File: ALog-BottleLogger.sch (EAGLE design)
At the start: 103 parts, among them IC2 ATMEGA644M, J6 5.5x2.1mm Barrel, Q1 220mA/50V/3.5Ω, Q4 4.3A/20V/54mΩ, Q5 4.3A/20V/54mΩ, Q6 4.3A/20V/54mΩ, Q7 4.3A/20V/54mΩ, Q8 220mA/50V/3.5Ω, Q9 220mA/50V/3.5Ω, U2 FT231X-Q

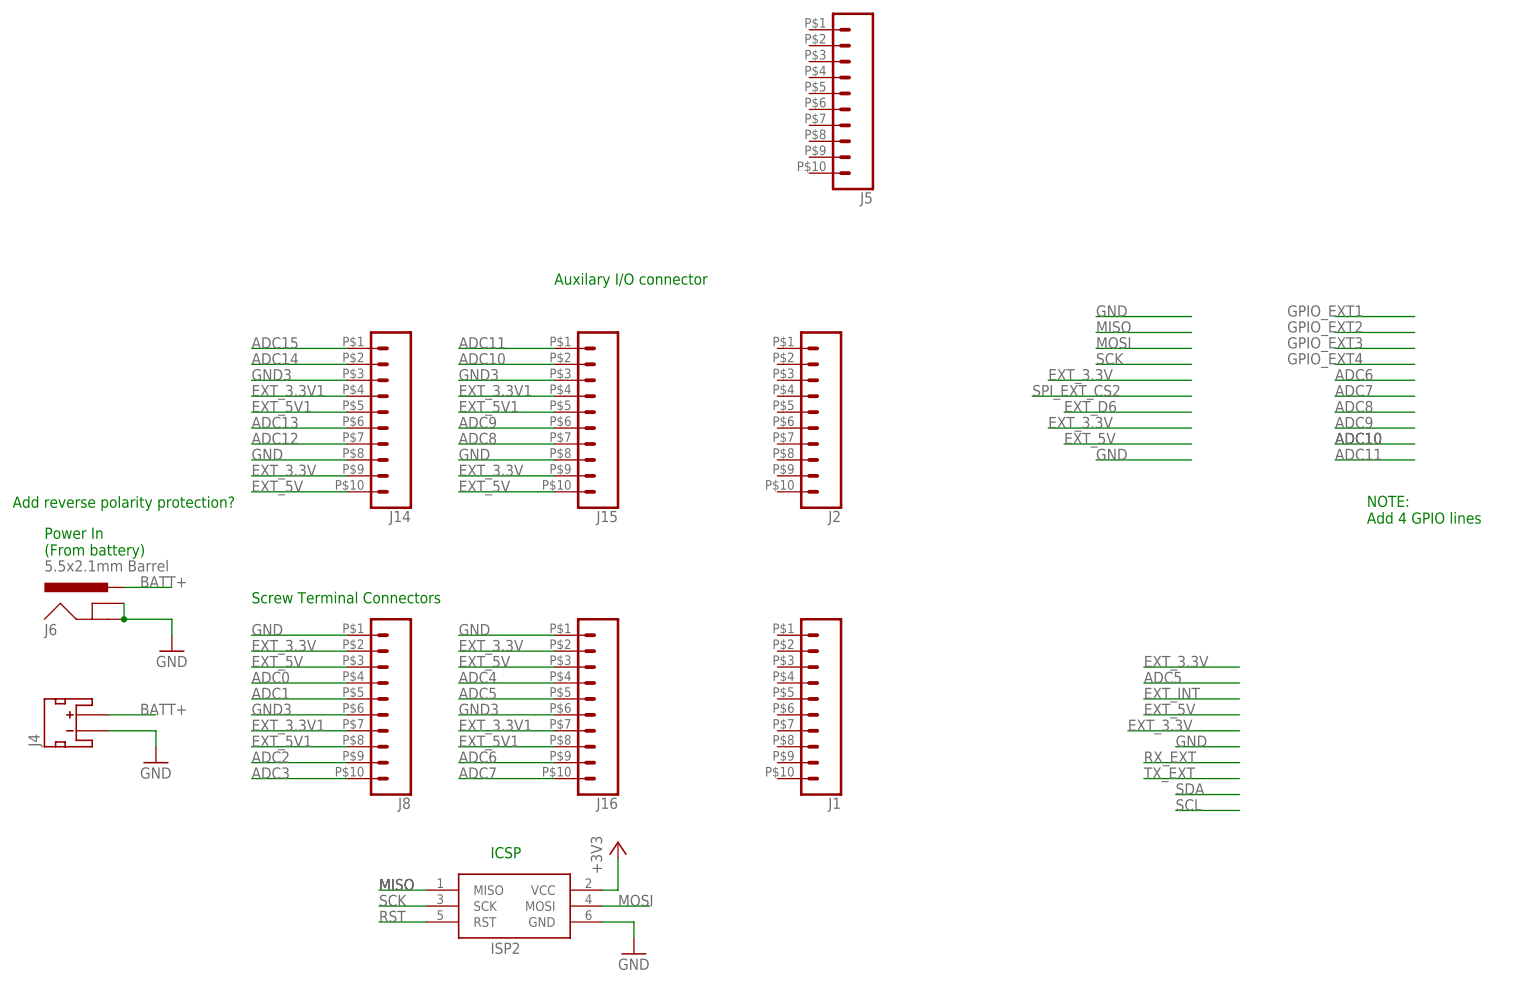
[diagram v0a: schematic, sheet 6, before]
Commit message: progress
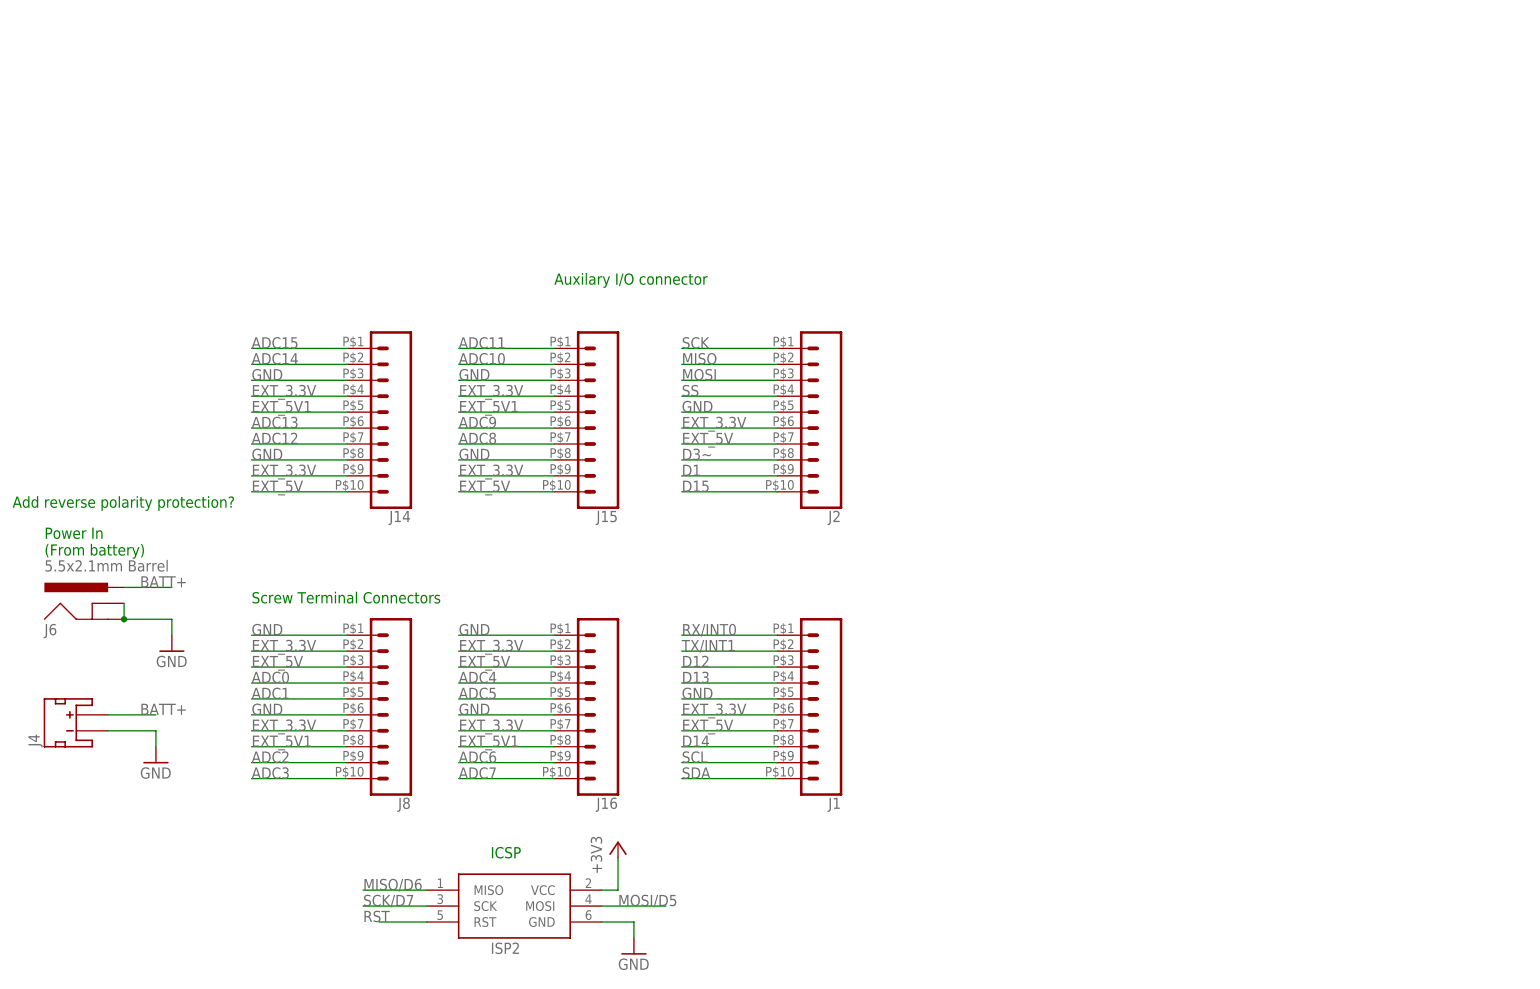
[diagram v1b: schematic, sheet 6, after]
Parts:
- removed J5: (no value), SparkFun-Connectors:CONN_10
- removed LED: (no value), SparkFun-LED:LED1206
- removed R_LED: 220, resistor:R-US_R0603
- added LED3: (no value), SparkFun-LED:LED1206
- added R_LED1: 220, resistor:R-US_R0603
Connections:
- net 26 renamed SD-VCC_CTRL
- net 27 renamed D19
- net 29 renamed D21
- net 3 renamed D3
- net SS/4 renamed SS/D4
- removed net 0: IC2.(PCINT8/XCK0/T0)PB0
- removed net 1: IC2.(PCINT9/CLKO/T1)PB1
- removed net 28: IC2.(PCINT20/TDO)PC4
- removed net 30: IC2.(PCINT22/TOSC1)PC6
- removed net EXT_3.3V1: J14.4, J15.4, J16.7, J8.7
- removed net GND3: J14.3, J15.3, J16.6, J8.6
- removed net LED: IC2.(PCINT31/OC2A)PD7, R_LED.1
- removed net LED+: LED.A, R_LED.2
- removed net MISO/6: IC2.(PCINT14/MISO)PB6
- removed net MOSI/5: IC2.(PCINT13/MOSI)PB5
- removed net SCK/7: IC2.(PCINT15/SCK)PB7
- new net D1: IC2.(PCINT9/CLKO/T1)PB1, J2.9
- new net D12: IC2.(PCINT28/OC1B)PD4, J1.3
- new net D13: IC2.(PCINT29/OC1A)PD5, J1.4
- new net D14: IC2.(PCINT30/OC2B/ICP)PD6, J1.8
- new net D15: IC2.(PCINT31/OC2A)PD7, J2.10
- new net D3~: J2.8
- new net LED+1: LED3.A, R_LED1.2
- new net MISO/D6: IC2.(PCINT14/MISO)PB6, ISP2.MISO
- new net MOSI/D5: IC2.(PCINT13/MOSI)PB5, ISP2.MOSI
- new net N$5: IC2.(PCINT8/XCK0/T0)PB0, R_LED1.1
- new net SCK/D7: IC2.(PCINT15/SCK)PB7, ISP2.SCK
- new net SS: J2.4
- net 3.3V_EXT_CTRL: now also IC2.(PCINT22/TOSC1)PC6; no longer IC2.(PCINT30/OC2B/ICP)PD6
- net 5V_EXT_CTRL: now also IC2.(PCINT20/TDO)PC4; no longer IC2.(PCINT29/OC1A)PD5
- net EXT_3.3V: now also J1.6, J14.4, J15.4, J16.7, J2.6, J8.7
- net EXT_5V: now also J1.7, J2.7
- net GND: now also J1.5, J14.3, J15.3, J16.6, J2.5, J8.6, LED3.C; no longer LED.C
- net MISO: now also J2.2; no longer ISP2.MISO
- net MOSI: now also J2.3; no longer ISP2.MOSI
- net RX/INT0: now also J1.1
- net SCK: now also J2.1; no longer ISP2.SCK
- net SCL: now also J1.9
- net SDA: now also J1.10
- net SD_VCC_CTRL: no longer IC2.(PCINT28/OC1B)PD4
- net TX/INT1: now also J1.2
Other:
- note removed: "NOTE: Add 4 GPIO lines"
